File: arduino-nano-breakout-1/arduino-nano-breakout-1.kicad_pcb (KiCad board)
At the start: 2 copper layers, 7 x 7 mm, 4 parts, among them J1 PJ-002A, J2 Conn_01x03_Male, J4 Conn_01x08_Male

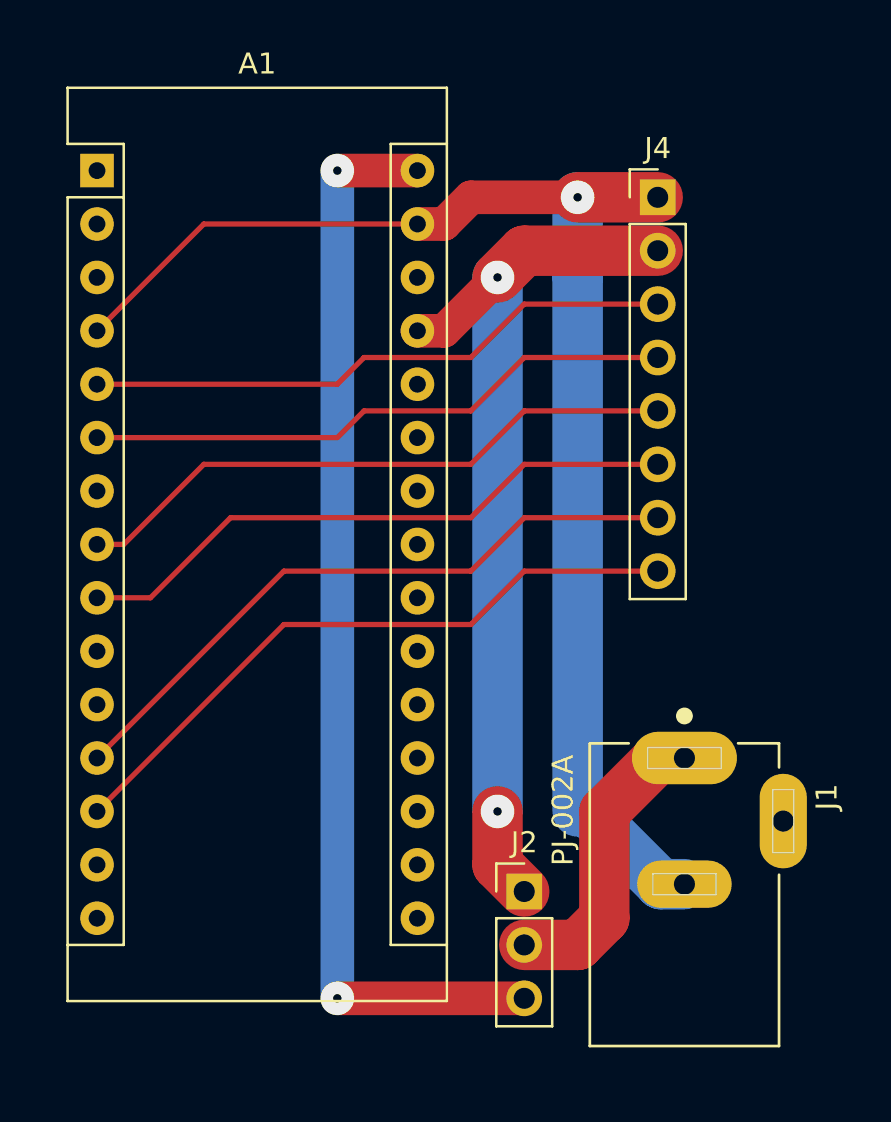
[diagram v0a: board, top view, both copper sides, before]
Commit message: move
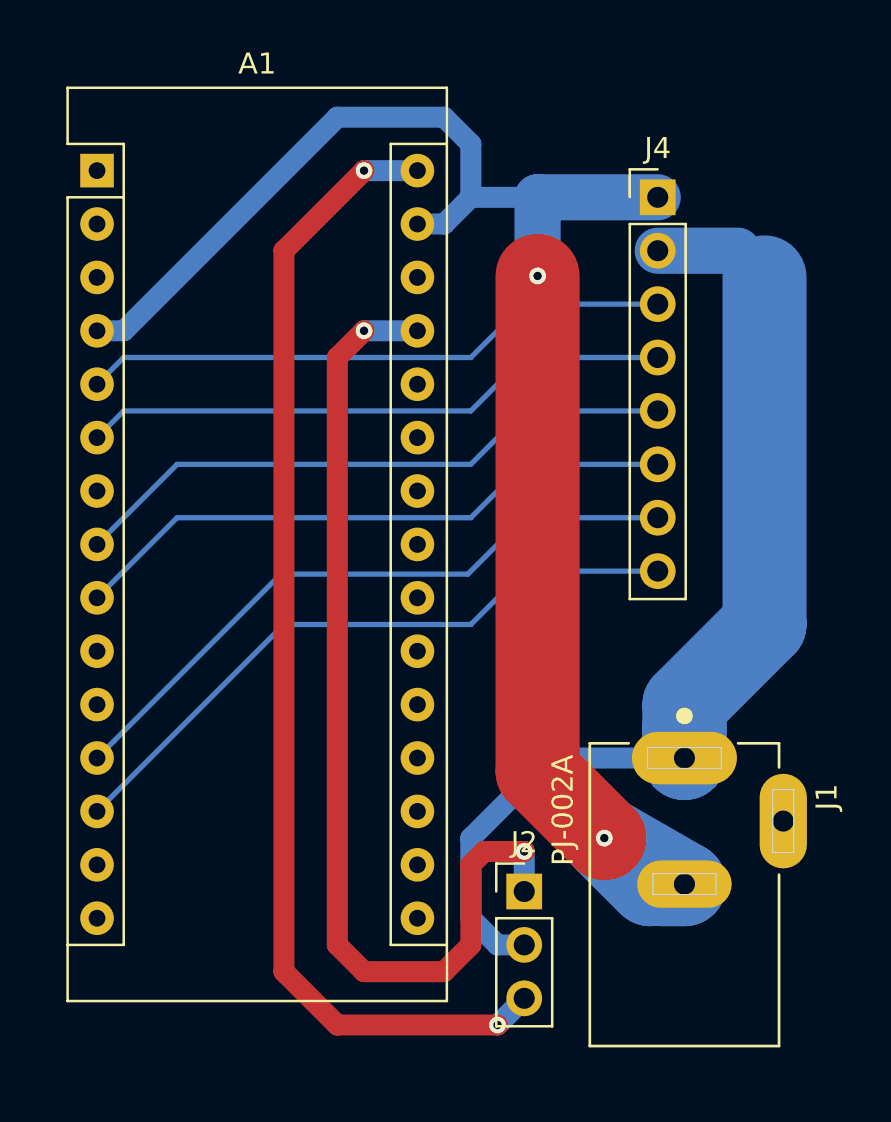
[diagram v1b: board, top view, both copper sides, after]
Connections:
- J4 pad 2: Net-(A1-Pad27) -> Net-(J1-Pad1)
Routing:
- net Net-(J1-Pad1): track 14.5 -> 51.3 mm
- net GND: track 65.4 -> 80.5 mm, vias 1 -> 2
- net Net-(A1-Pad27): track 42.7 -> 48.2 mm
- net Net-(A1-Pad30): track 52.1 -> 55.2 mm

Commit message: final piece?
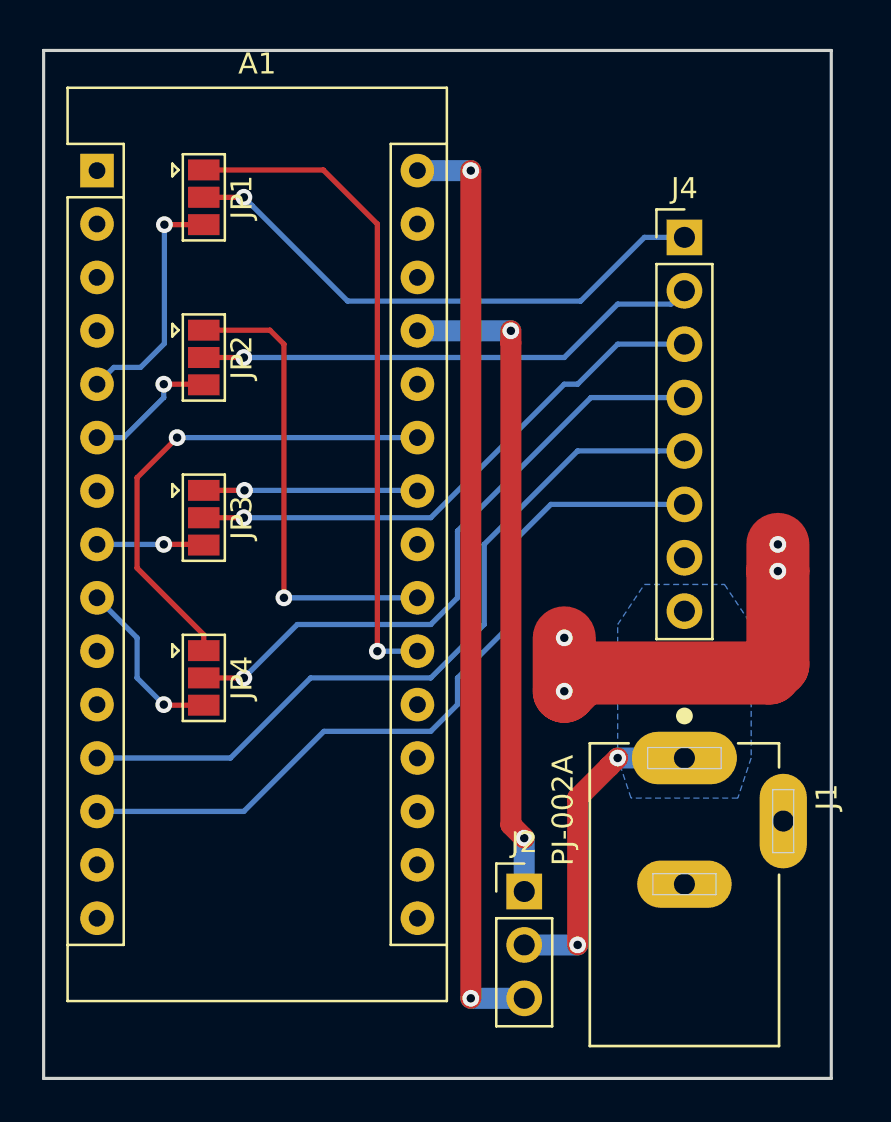
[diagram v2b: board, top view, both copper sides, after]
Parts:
- added JP1: SolderJumper_3_Open, Jumper:SolderJumper-3_P1.3mm_Open_Pad1.0x1.5mm, F.Cu at (134.6, 77.5)
- added JP2: SolderJumper_3_Open, Jumper:SolderJumper-3_P1.3mm_Open_Pad1.0x1.5mm, F.Cu at (134.6, 85.1)
- added JP3: SolderJumper_3_Open, Jumper:SolderJumper-3_P1.3mm_Open_Pad1.0x1.5mm, F.Cu at (134.6, 92.7)
- added JP4: SolderJumper_3_Open, Jumper:SolderJumper-3_P1.3mm_Open_Pad1.0x1.5mm, F.Cu at (134.6, 100.3)
- J1: footprint CUI_PJ-002A -> SS_connectors:CUI_PJ-002A
- moved J4 2.29 mm to (157.5, 79.4)
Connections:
- A1 pad 1: Net-(A1-Pad1) -> (no net)
- A1 pad 10: Net-(A1-Pad10) -> (no net)
- A1 pad 11: Net-(A1-Pad11) -> (no net)
- A1 pad 14: Net-(A1-Pad14) -> (no net)
- A1 pad 15: Net-(A1-Pad15) -> (no net)
- A1 pad 16: Net-(A1-Pad16) -> (no net)
- A1 pad 17: Net-(A1-Pad17) -> (no net)
- A1 pad 18: Net-(A1-Pad18) -> (no net)
- A1 pad 19: Net-(A1-Pad19) -> (no net)
- A1 pad 2: Net-(A1-Pad2) -> (no net)
- A1 pad 20: Net-(A1-Pad20) -> (no net)
- A1 pad 23: Net-(A1-Pad23) -> (no net)
- A1 pad 26: Net-(A1-Pad26) -> (no net)
- A1 pad 28: Net-(A1-Pad28) -> (no net)
- A1 pad 3: Net-(A1-Pad3) -> (no net)
- A1 pad 7: Net-(A1-Pad7) -> (no net)
- J1 pad 3: Net-(J1-Pad3) -> (no net)
- J4 pad 1: GND -> Net-(J4-Pad1)
- J4 pad 2: Net-(J1-Pad1) -> Net-(J4-Pad2)
- J4 pad 3: IO2 -> Net-(J4-Pad3)
- J4 pad 4: IO3 -> Net-(J4-Pad4)
- J4 pad 5: IO5 -> IO9
- J4 pad 6: IO6 -> IO10
- J4 pad 7: IO9 -> GND
- J4 pad 8: IO10 -> Net-(J1-Pad1)
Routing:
- net GND: track 80.5 -> 18.9 mm, vias 2 -> 4
- net Net-(J1-Pad1): track 51.3 -> 15.4 mm, vias 0 -> 2
- net Net-(A1-Pad21): track 0.00 -> 31.5 mm, vias 0 -> 1
- net Net-(J4-Pad4): track 0.00 -> 30.2 mm, vias 0 -> 1
- net Net-(J4-Pad3): track 0.00 -> 26.3 mm, vias 0 -> 1
- net Net-(J4-Pad1): track 0.00 -> 26.2 mm, vias 0 -> 1
- net IO5: track 29.3 -> 5.09 mm, vias 0 -> 1
- net Net-(J4-Pad2): track 0.00 -> 24.2 mm, vias 0 -> 1
- net Net-(A1-Pad25): track 0.00 -> 23.7 mm, vias 0 -> 1
- net Net-(A1-Pad22): track 0.00 -> 22.5 mm, vias 0 -> 1
- net IO3: track 28.2 -> 6.52 mm, vias 0 -> 1
- net IO6: track 29.3 -> 8.31 mm, vias 0 -> 1
- net Net-(A1-Pad27): track 48.2 -> 31.4 mm
- net IO2: track 28.2 -> 11.5 mm, vias 0 -> 1
- net Net-(A1-Pad30): track 55.2 -> 44.5 mm
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- added copper zone on B.Cu, net GND
- added copper zone on B.Cu, net Net-(J1-Pad1)
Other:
- board size 7 x 7 mm -> 37.5 x 48.9 mm
